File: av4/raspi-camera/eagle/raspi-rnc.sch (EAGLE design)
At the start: 42 parts, among them J1 RP-REV2-MOAR, J2 ROCKETNET-CONNECTOR-16M, T1 ALT4532, T2 ALT4532, U1 LMZ12001, U2 LMZ12001

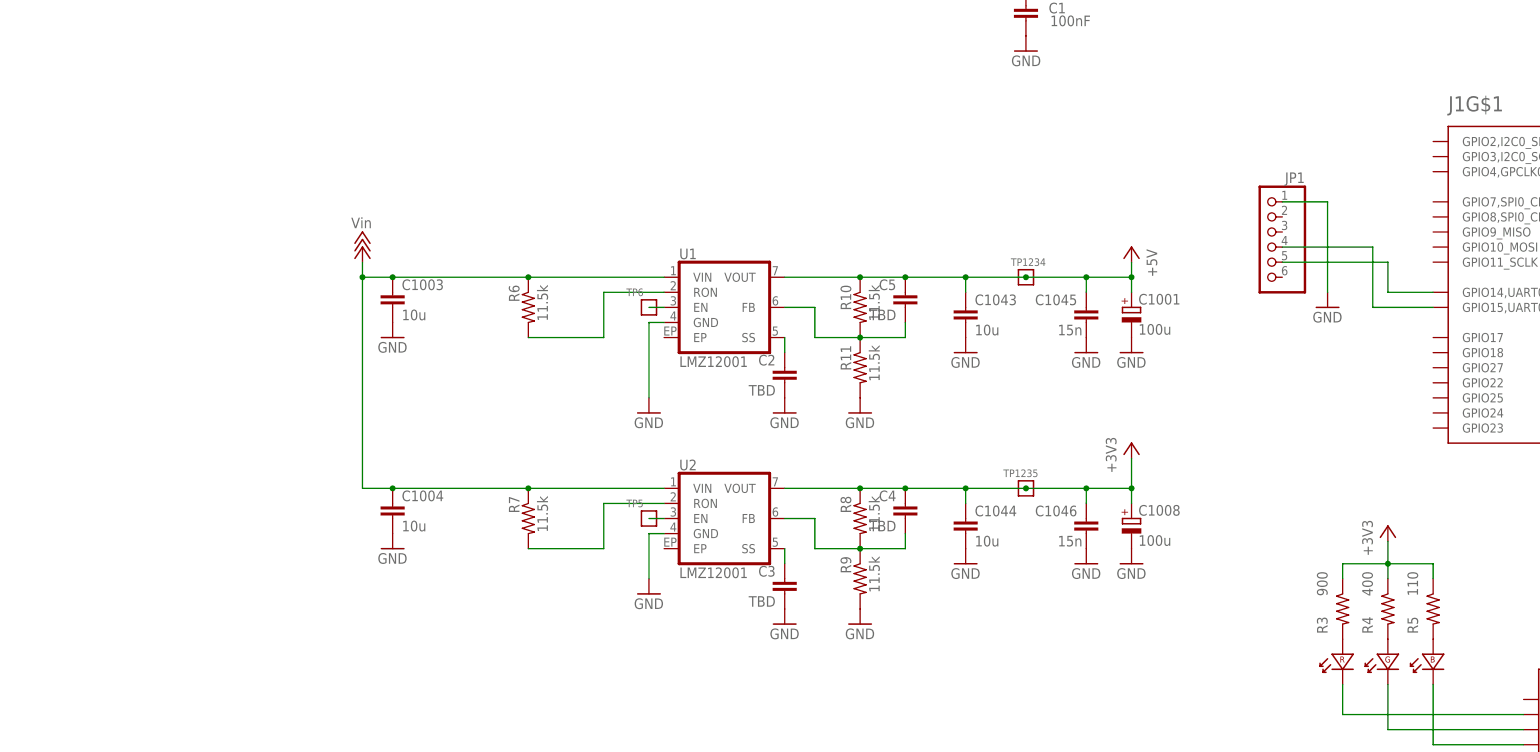
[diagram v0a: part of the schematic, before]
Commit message: Completed RPi daughterboard layout.
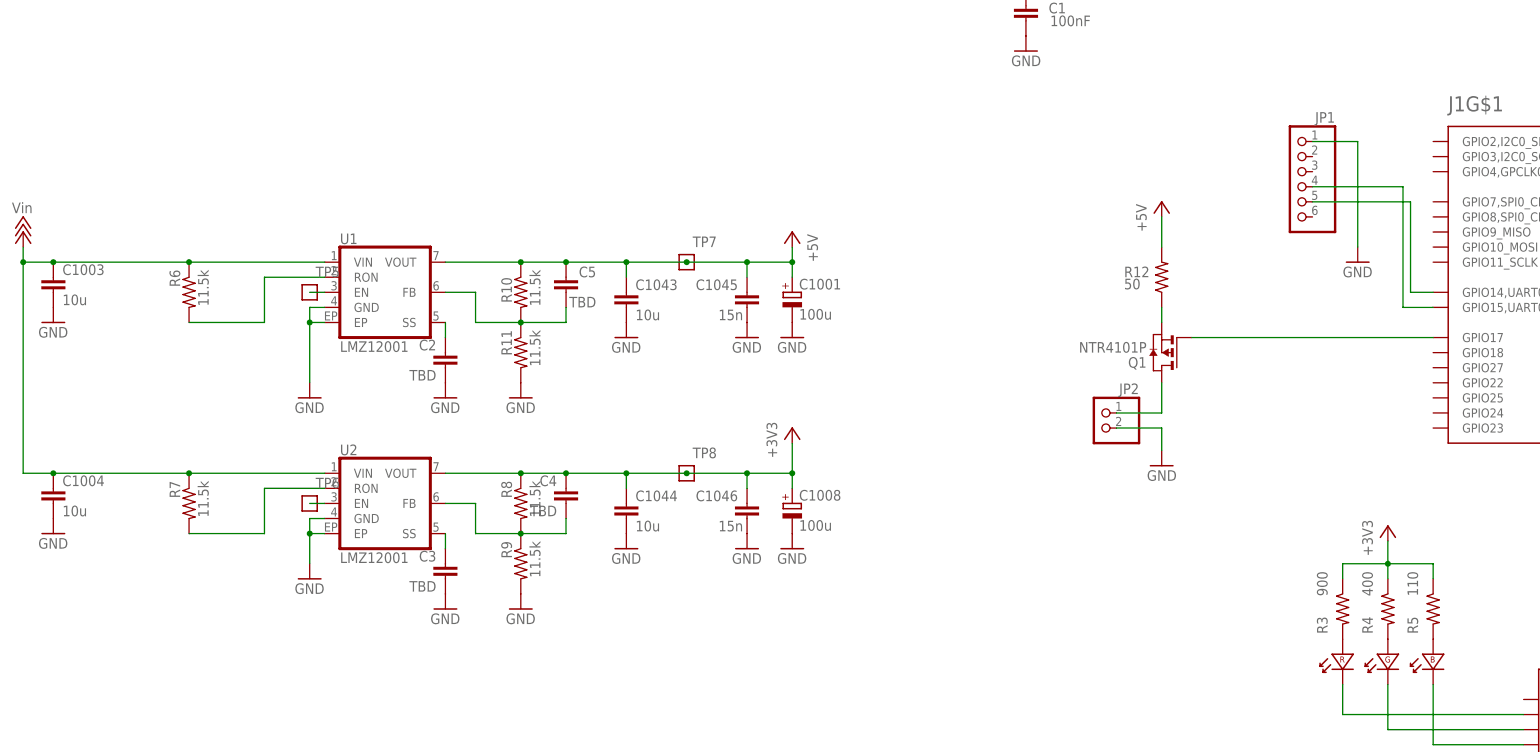
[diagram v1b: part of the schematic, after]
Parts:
- removed TP1234, TP1235: TEST, tqm:TEST
- added JP2: (no value), pinhead:PINHD-1X2
- added Q1: NTR4101P, Tova:NTR4101P
- added R12: 50, rcl_custom:R-US_0603-B-NOSILK
- added TP7, TP8: TEST-POINT, apdm:TEST-POINT
- JP1: device pinhead:PINHD-1X6/90 -> pinhead:PINHD-1X6
- TP5, TP6: value TEST -> TEST-POINT; device tqm:TEST -> apdm:TEST-POINT
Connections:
- new net N$38: J1G$1.GPIO17, Q1.G
- new net N$39: JP2.1, Q1.D
- new net N$40: Q1.S, R12.1
- net +3V3: now also TP8.1; no longer TP1235.P$1
- net +5V: now also R12.2, TP7.1; no longer TP1234.P$1
- net GND: now also JP2.2, U1.EP, U2.EP
- net N$32: now also TP5.1; no longer TP6.P$1
- net N$33: now also TP6.1; no longer TP5.P$1
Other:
- moved on the sheet: C1001, C1003, C1004, C1008, C1043, C1044, C1045, C1046, C2, C3, C4, C5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
